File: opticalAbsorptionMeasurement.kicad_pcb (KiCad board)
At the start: 2 copper layers, 169 parts, among them J1 Conn_01x02_Male, J2 Conn_01x02_Male, J3 Conn_01x03_Male, J4 Conn_01x03_Male, J5 Conn_01x03_Male, J6 Conn_01x03_Male, J7 Conn_01x02_Male, J8 Conn_01x02_Male, J9 Conn_01x02_Male, Q1 J111, Q2 J111, Q3 J111, Q4 J111, U1 TEN5-0523, U10 ADR01, U11 OPA602AU, U12 OPA602AU, U13 OPA602AU, U14 OPA602AU, U15 OPA602AU, U16 OPA602AU, U19 OPA602AU, U2 OPA602AU, U20 OPA602AU, U21 OPA602AU, U22 OPA602AU, U23 OPA602AU, U24 OPA602AU, U3 OPA602AU, U6 L7812, U7 L7912, U8 OPA602AU, U9 OPA602AU

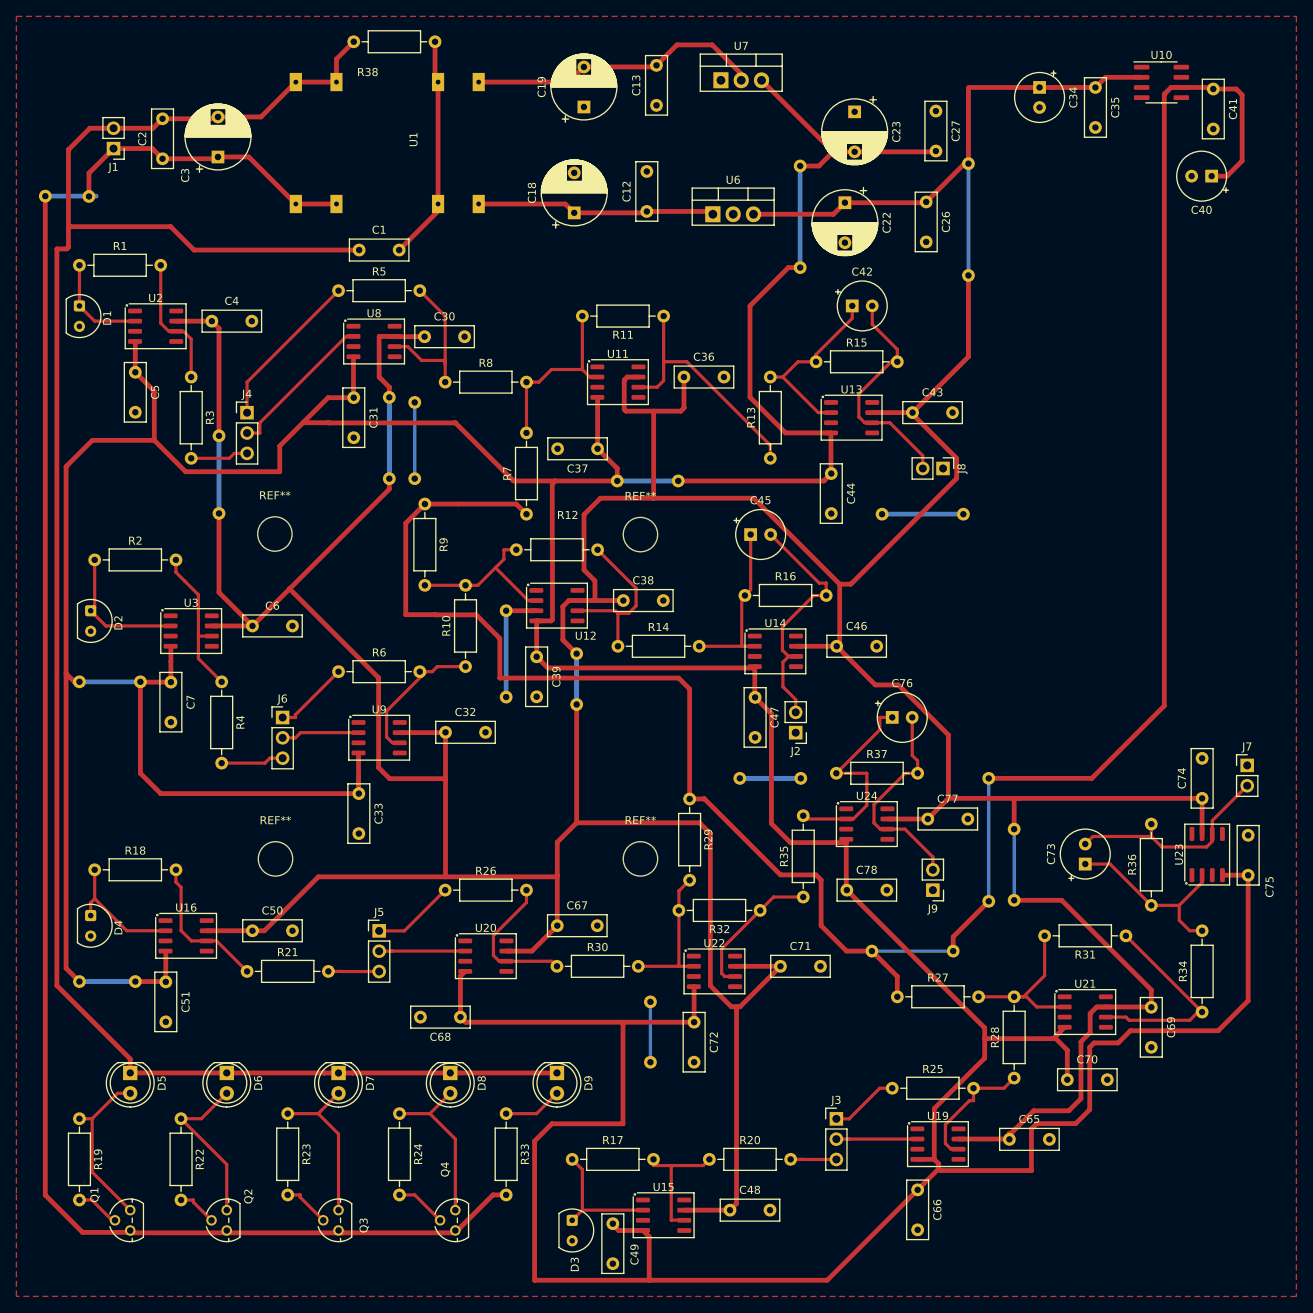
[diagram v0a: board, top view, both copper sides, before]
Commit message: update resistor
update resistor
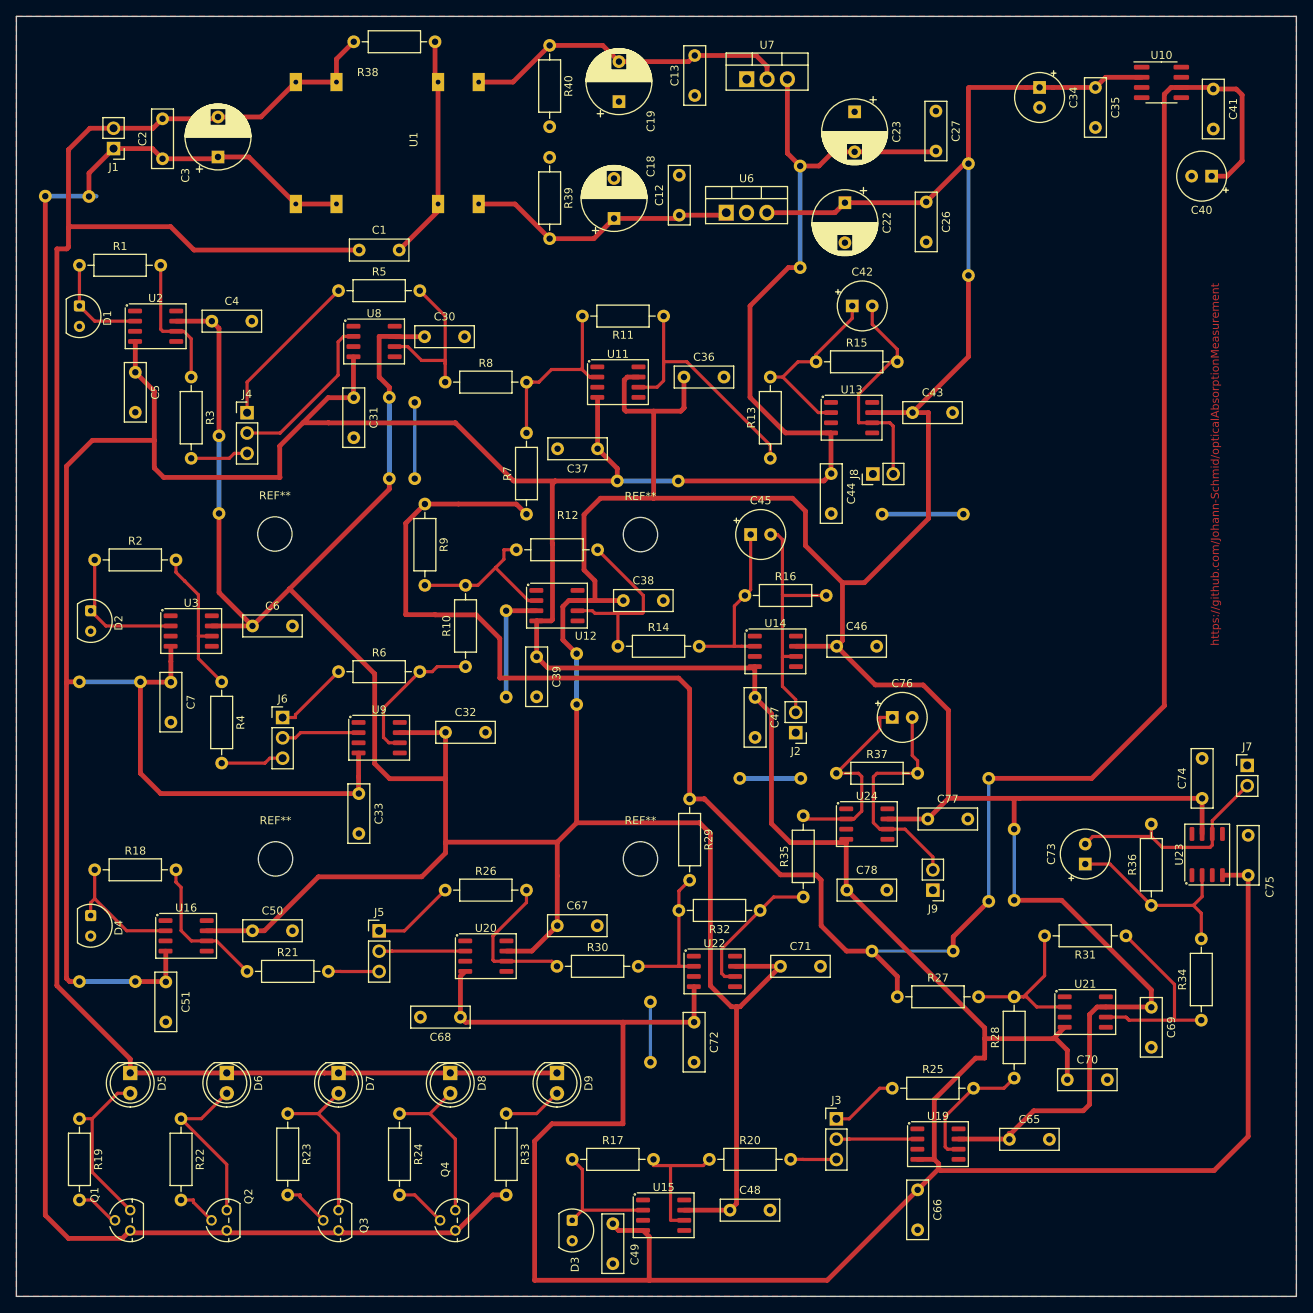
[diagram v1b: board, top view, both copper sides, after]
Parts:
- added R39: 10k, Resistor_THT:R_Axial_DIN0207_L6.3mm_D2.5mm_P10.16mm_Horizontal, F.Cu at (91.8, 71.6)
- added R40: 10k, Resistor_THT:R_Axial_DIN0207_L6.3mm_D2.5mm_P10.16mm_Horizontal, F.Cu at (91.8, 57.6)
- moved J8 8.80 mm to (132.2, 111.2), turned to 90 degrees
- moved C18 5.03 mm to (99.8, 79.2)
- moved C13 4.93 mm to (109.9, 63.9)
- moved C19 4.43 mm to (100.5, 64.6)
- moved C12 4.09 mm to (108.0, 78.8)
- moved U7 3.23 mm to (116.4, 61.8)
- moved U6 1.68 mm to (113.9, 78.5)
- moved R34 1.02 mm to (173.3, 179.5)
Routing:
- net -12V: track 742.1 -> 747.3 mm
- net -15V: track 37.0 -> 41.3 mm
- net +15V: track 29.9 -> 34.1 mm
- net V3: track 27.4 -> 29.5 mm
- net +5V: track 232.2 -> 234.3 mm
- net Net-(R12-Pad1): track 21.0 -> 22.7 mm
- net RW2: track 19.1 -> 20.7 mm
- net Net-(C76-Pad1): track 27.4 -> 26.3 mm
- net +12V: track 714.7 -> 715.8 mm
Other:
- board outline added: 160 x 160 mm
- board text added: "https://github.com/Johann-Schmid/opticalAbsorptionMeasurement"
